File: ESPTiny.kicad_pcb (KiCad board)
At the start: 2 copper layers, 33 x 26.4 mm, 18 parts, among them J1 Conn_01x10_Male, J2 Conn_01x10_Male, J3 Conn_01x04_Male, U1 ESP-01v090, U2 ATtiny84-20PU, U3 MCP1700-3302E_TO92

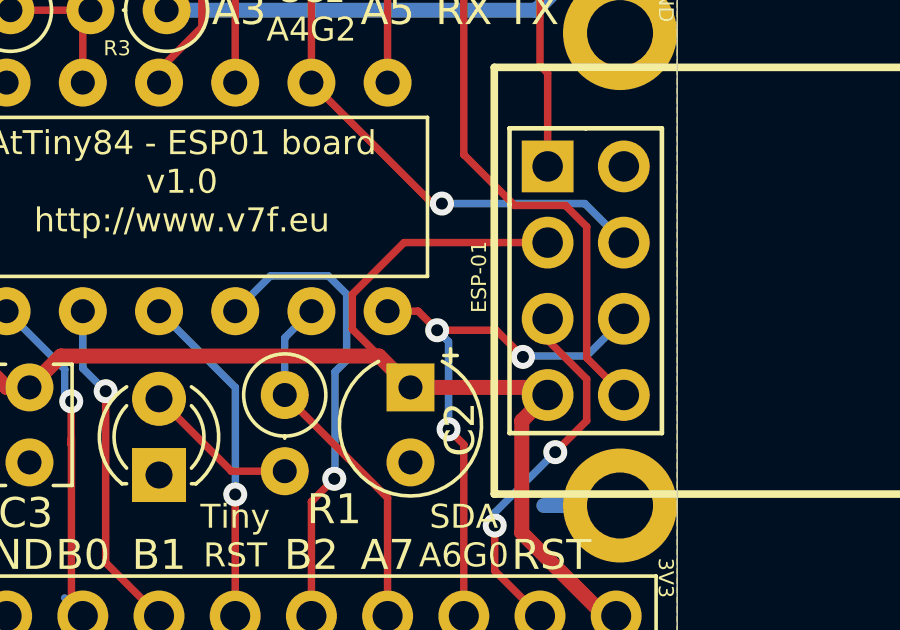
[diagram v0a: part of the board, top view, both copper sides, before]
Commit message: Copper fill
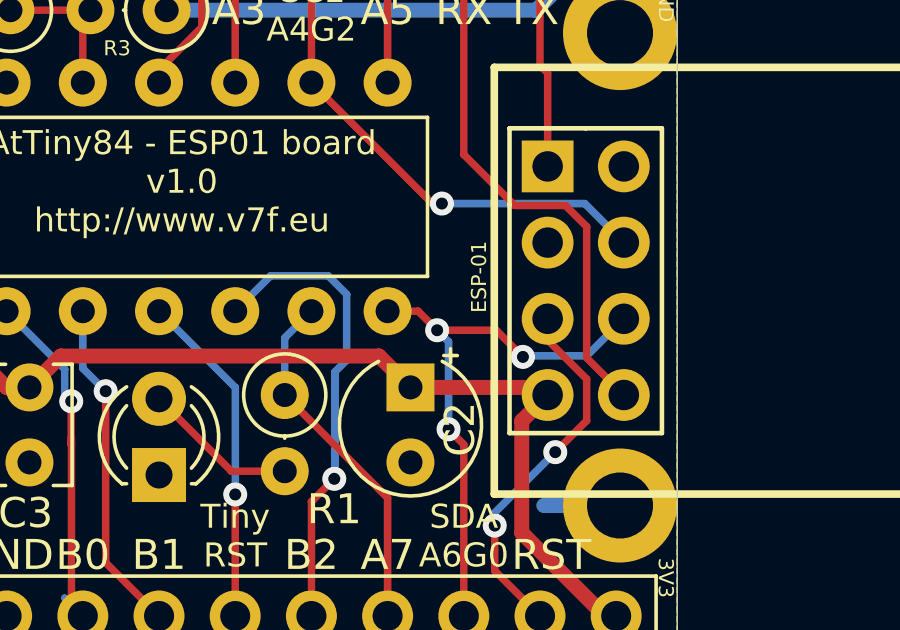
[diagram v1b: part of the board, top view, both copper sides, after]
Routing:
- net +3V3: track 56.2 -> 45.1 mm
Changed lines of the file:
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@@
     (thickness 1.6)
     (drawings 49)
-    (tracks 154)
+    (tracks 150)
     (zones 0)
     (modules 18)
@@
   (segment (start 43.942 61.722) (end 47.244 65.024) (width 0.5) (layer F.Cu) (net 2))
   (segment (start 43.942 60.706) (end 43.942 61.722) (width 0.5) (layer F.Cu) (net 2))
-  (segment (start 61.308999 55.466999) (end 63.246 57.404) (width 0.25) (layer F.Cu) (net 2))
-  (segment (start 61.308999 54.299999) (end 61.308999 55.466999) (width 0.25) (layer F.Cu) (net 2))
-  (segment (start 63.030998 52.578) (end 61.308999 54.299999) (width 0.25) (layer F.Cu) (net 2))
-  (segment (start 67.818 52.578) (end 63.030998 52.578) (width 0.25) (layer F.Cu) (net 2))
   (segment (start 43.528999 48.419001) (end 43.434 48.514) (width 0.25) (layer F.Cu) (net 3))
   (segment (start 43.022999 48.102999) (end 43.434 48.514) (width 0.5) (layer F.Cu) (net 3))
@@
   )
   (zone (net 2) (net_name +3V3) (layer F.Cu) (hatch edge 0.508)
+    (priority 1)
     (connect_pads (clearance 0.508))
     (min_thickness 0.254)
